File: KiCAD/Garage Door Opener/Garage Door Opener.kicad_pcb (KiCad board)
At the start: 2 copper layers, 57 x 57 mm, 10 parts, among them J1 Screw_Terminal_01x03, J3 Conn_01x02_Pin, K1 JQC-3FF-S-Z, Q1 S8550, SW1 SW_Push_Dual, U1 YD-ESP32-S3

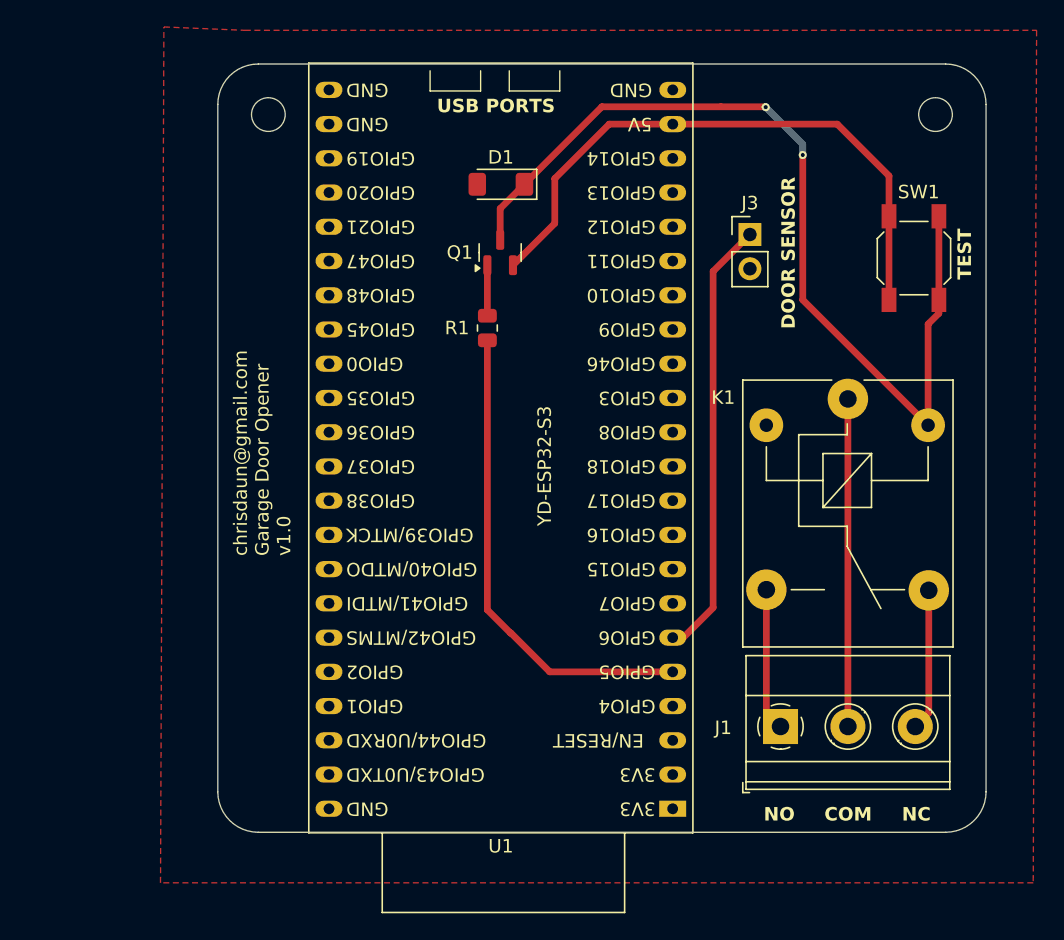
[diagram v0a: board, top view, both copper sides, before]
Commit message: Updated board design
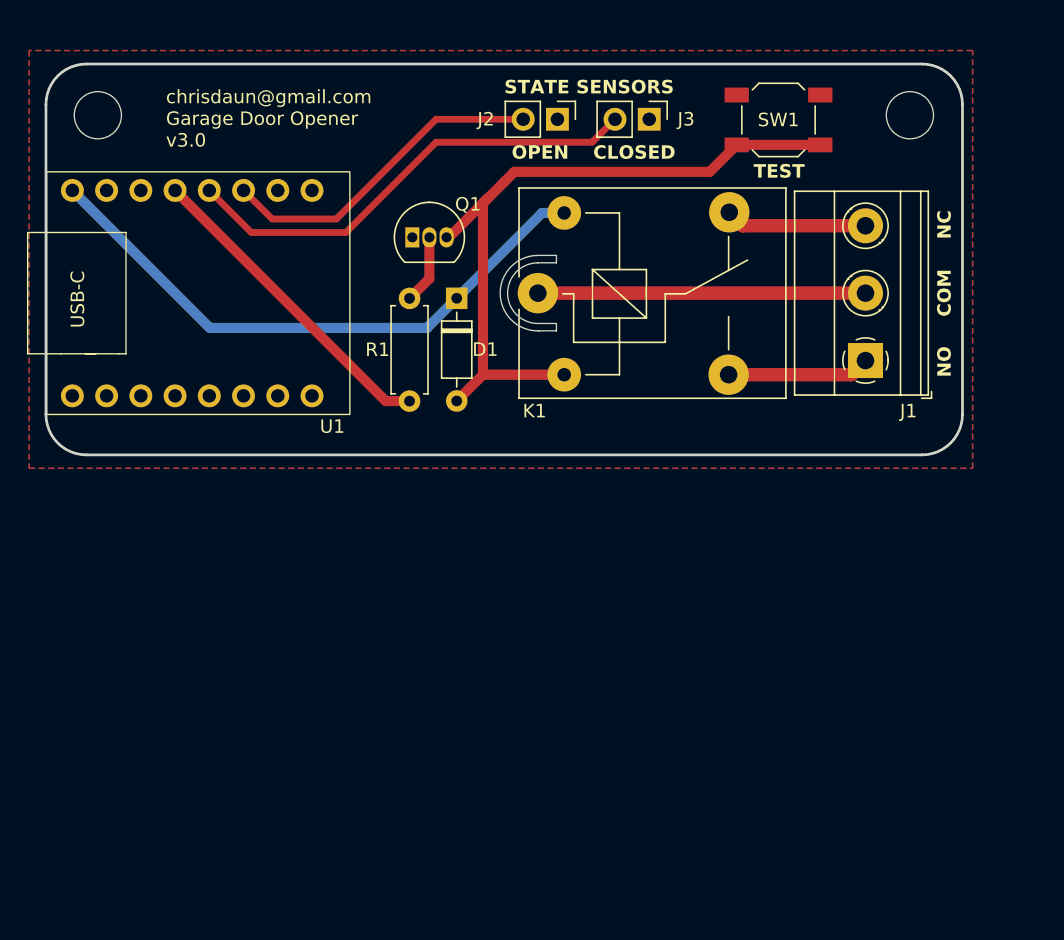
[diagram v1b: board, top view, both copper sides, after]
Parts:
- removed REF** (x2): MountingHole_2.5mm, MountingHole:MountingHole_2.5mm
- added H1: MountingHole, MountingHole:MountingHole_3.5mm, F.Cu at (55.1, 54.8)
- added H2: MountingHole, MountingHole:MountingHole_3.5mm, F.Cu at (115.3, 54.8)
- added J2: Conn_01x02_Pin, Connector_PinHeader_2.54mm:PinHeader_1x02_P2.54mm_Vertical, F.Cu at (89.2, 55.1)
- D1: footprint Diode_SMD:D_MiniMELF -> Diode_THT:D_DO-35_SOD27_P7.62mm_Horizontal
- Q1: value S8550 -> PN2222A; footprint Package_TO_SOT_SMD:SOT-23 -> Package_TO_SOT_THT:TO-92_Inline
- R1: footprint Resistor_SMD:R_0805_2012Metric -> Resistor_THT:R_Axial_DIN0207_L6.3mm_D2.5mm_P7.62mm_Horizontal
- SW1: value SW_Push_Dual -> SW_Push
- U1: value YD-ESP32-S3 -> ~; footprint Custom Footprints:YD-ESP32-S3 -> esp32-homespan-garagedoor-opener:ESP32-C3 Super Micro
- moved U1 52.5 mm to (62.5, 68.0), turned to 90 degrees
- moved J1 27.9 mm to (112.1, 73.0), turned to 90 degrees
- moved K1 24.3 mm to (87.8, 68.0), turned to 0 degrees
- moved SW1 14.4 mm to (105.6, 55.1), turned to 180 degrees
- moved J3 11.4 mm to (96.0, 55.1), turned to -90 degrees
- moved D1 9.07 mm to (81.7, 68.4), turned to -90 degrees
- moved R1 7.92 mm to (78.2, 76.0)
- moved Q1 6.62 mm to (78.4, 63.9), turned to 0 degrees
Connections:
- D1 pad 1: Net-(D1-K) -> +5V
- D1 pad 2: GND -> Net-(D1-A)
- J3 pad 1: Net-(J3-Pin_1) -> GND
- J3 pad 2: GND -> Net-(J3-Pin_2)
- K1 pad 1: Net-(D1-K) -> +5V
- K1 pad 2: GND -> Net-(D1-A)
- Q1 pad 1: Net-(Q1-E) -> GND
- Q1 pad 2: +5V -> Net-(Q1-B)
- Q1 pad 3: Net-(D1-K) -> Net-(D1-A)
- R1 pad 1: Net-(U1-GPIO5/ADC1_CH4) -> Net-(U1-GPIO_4)
- R1 pad 2: Net-(Q1-E) -> Net-(Q1-B)
- SW1 pad 1: +5V -> Net-(D1-A)
- SW1 pad 2: Net-(D1-K) -> GND
- U1 pad 2: unconnected-(U1-3V3-Pad1)_1 -> Net-(J2-Pin_2)
- U1 pad 21: +5V -> unconnected-(U1-GPIO_21-Pad21)
- U1 pad 3: unconnected-(U1-CHIP_PU-Pad3) -> Net-(J3-Pin_2)
- U1 pad 4: unconnected-(U1-GPIO4/ADC1_CH3-Pad4) -> Net-(U1-GPIO_4)
- U1 pad 5: Net-(U1-GPIO5/ADC1_CH4) -> unconnected-(U1-GPIO_5-Pad5)
- U1 pad 6: Net-(J3-Pin_1) -> unconnected-(U1-GPIO_6-Pad6)
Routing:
- net Net-(D1-K): track 69.6 -> 0.00 mm, vias 2 -> 0
- net Net-(D1-A): track 0.00 -> 53.3 mm
- net Net-(U1-GPIO5/ADC1_CH4): track 35.7 -> 0.00 mm
- net Net-(J3-Pin_2): track 0.00 -> 34.9 mm
- net Net-(J3-Pin_1): track 32.7 -> 0.00 mm
- net Net-(J2-Pin_2): track 0.00 -> 24.7 mm
- net Net-(U1-GPIO_4): track 0.00 -> 23.9 mm
- net Net-(Q1-B): track 0.00 -> 5.14 mm
- net Net-(Q1-E): track 3.75 -> 0.00 mm
- net +5V: track 45.2 -> 44.2 mm
- added copper zone on B.Cu, net GND
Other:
- board size 57 x 57 mm -> 68 x 29 mm
- board text added: "CLOSED"
- board text added: "OPEN"
- board text added: "STATE SENSORS"
- board text added: "chrisdaun@gmail.com Garage Door Opener v3.0"
- board text removed: "DOOR SENSOR"
- board text removed: "USB PORTS"
- board text removed: "chrisdaun@gmail.com Garage Door Opener v1.0"
